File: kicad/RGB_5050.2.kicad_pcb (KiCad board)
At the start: 2 copper layers, 15.2 x 15.2 mm, 6 parts, among them J1 Conn_01x03_Female, J2 Conn_01x03_Female, J3 Conn_01x03_Female, J4 Conn_01x03_Female

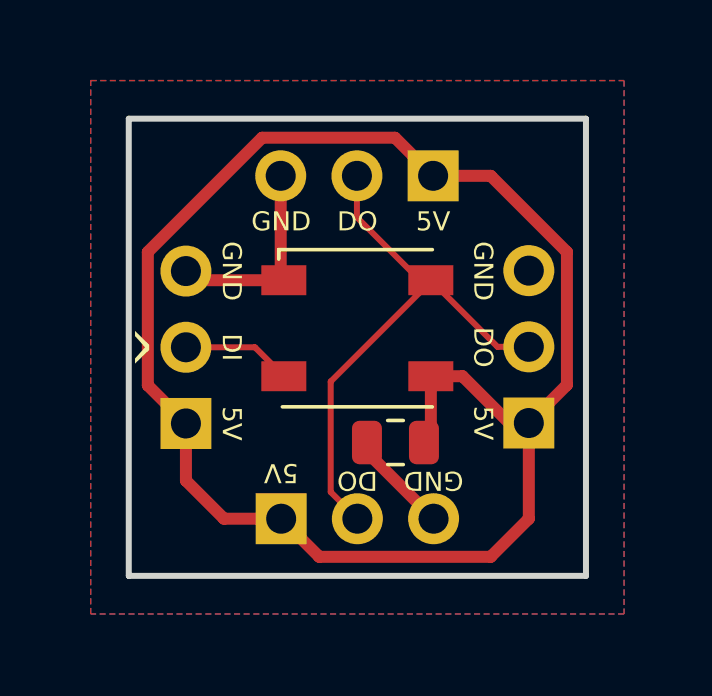
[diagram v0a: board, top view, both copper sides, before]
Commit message: v1 adjustments
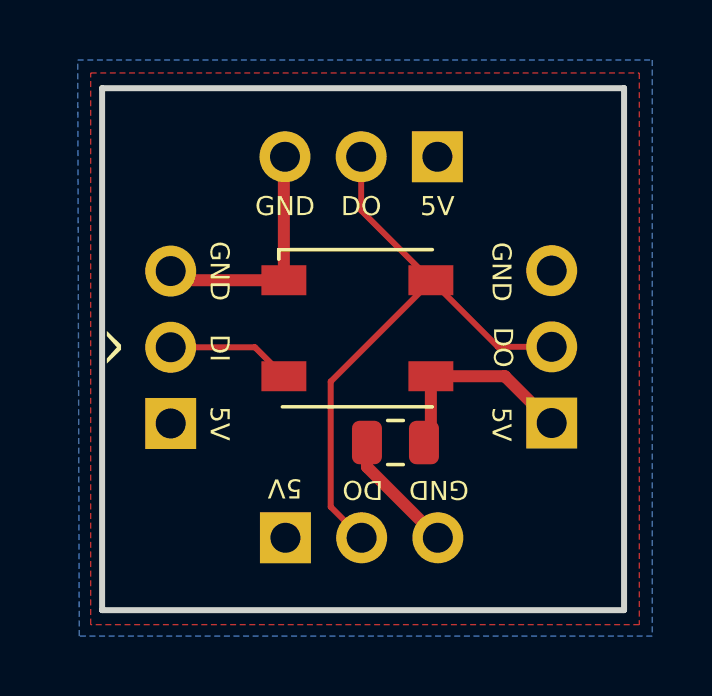
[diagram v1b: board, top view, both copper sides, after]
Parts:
- added G***: LOGO, LOGO, B.Cu at (131.9, 103.2)
- moved J4 0.76 mm to (140.5, 107.3)
- moved J2 0.65 mm to (136.7, 98.4)
- moved J3 0.65 mm to (131.6, 111.1)
- moved J1 0.51 mm to (127.8, 107.3)
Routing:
- net +5V: track 53.9 -> 6.98 mm
- net DOUT: track 18.6 -> 20.4 mm
- net GND: track 10.4 -> 12.2 mm
- net DIN: track 3.66 -> 4.17 mm
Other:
- board size 15.2 x 15.2 mm -> 17.4 x 17.4 mm
- board text added: "github.com/ jedp/RGB-5050-2"
